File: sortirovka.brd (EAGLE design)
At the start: 160 x 100 mm, 19 parts, among them U1 MAX3485CSA, X1 PI3-CON, X2 MKDSN1,5/2-5,08, X3 MKDSN1,5/4-5,08, X4 MKDSN1,5/2-5,08

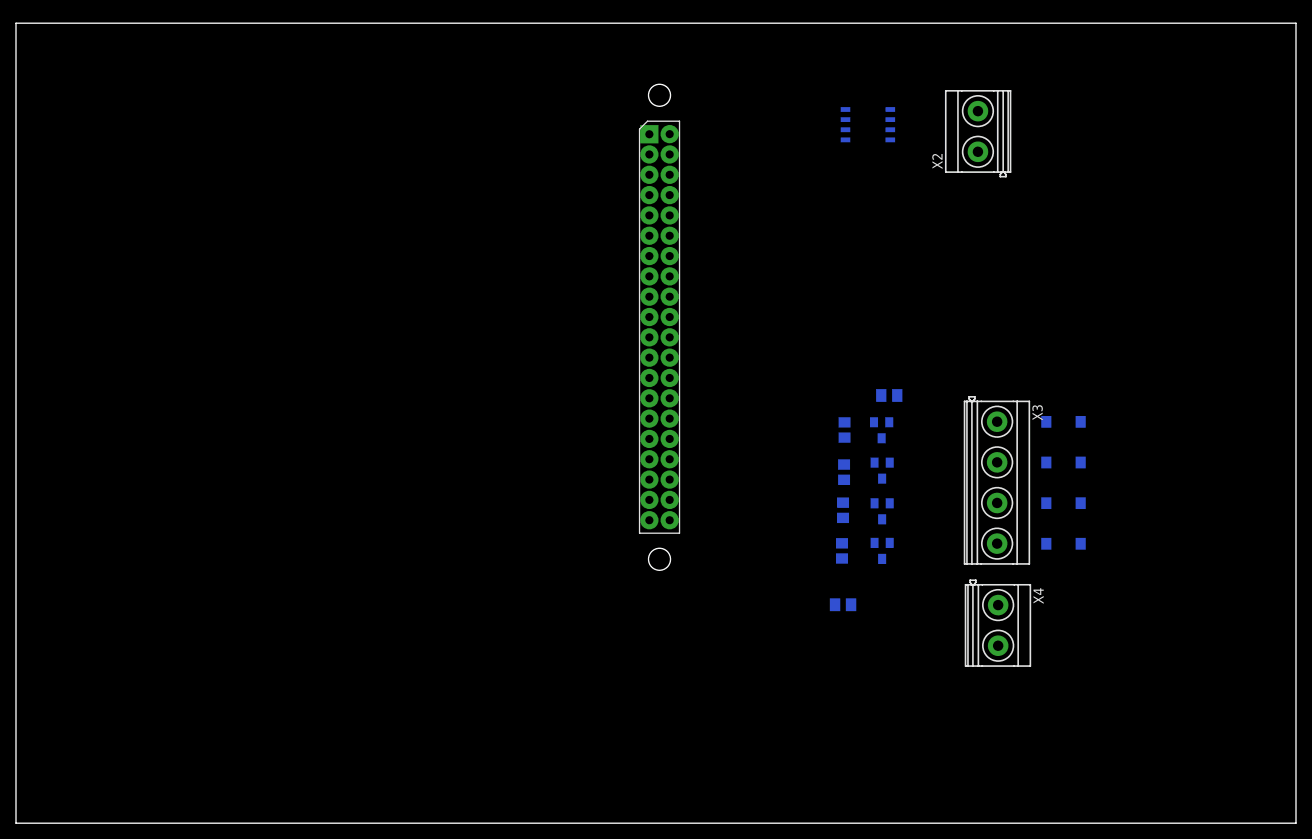
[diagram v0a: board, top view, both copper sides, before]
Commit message: rev1
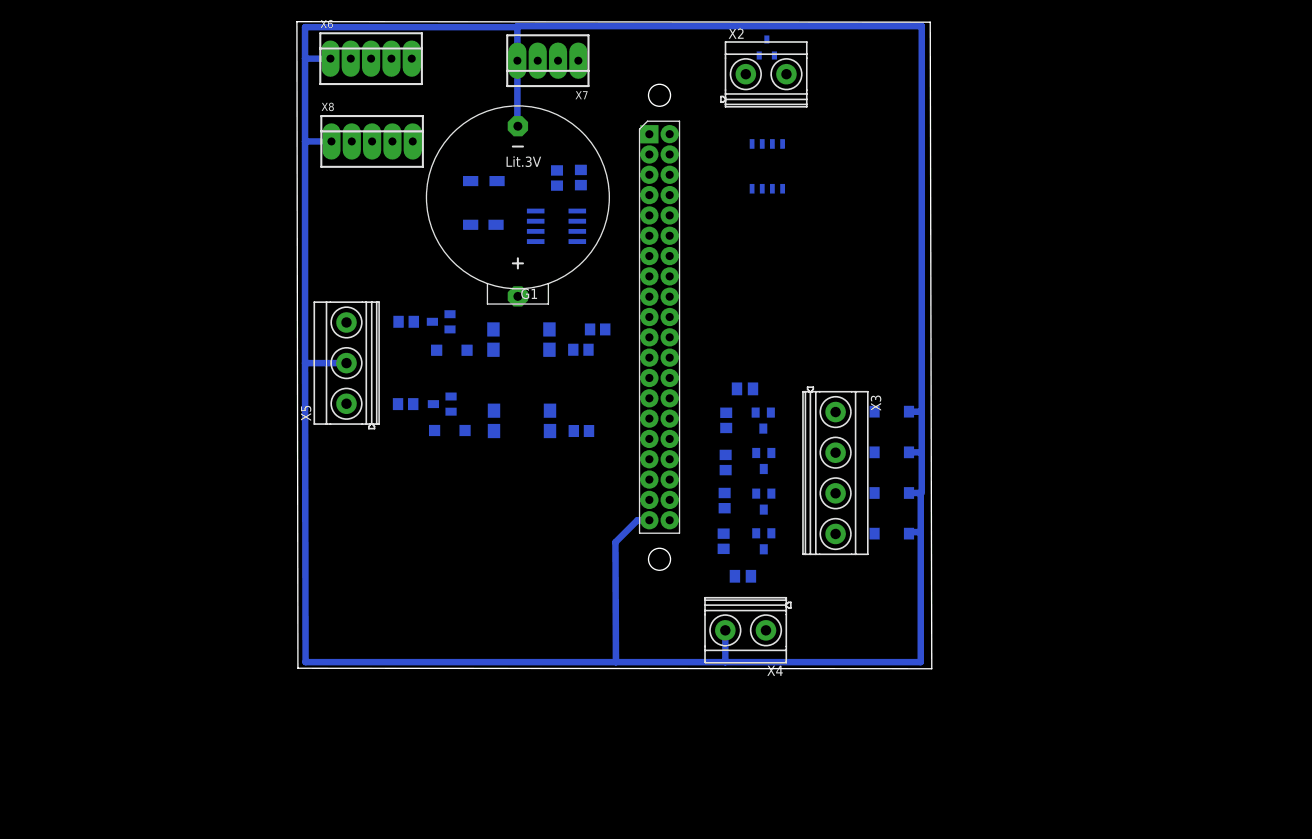
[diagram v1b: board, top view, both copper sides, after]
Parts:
- added D5, D6: BAV199, diode:SOT23
- added G1: CR2032H, MyLib:CR2032H
- added IC1: DS1307Z, MyLib:SOIC8
- added OC1, OC2: (no value), MyLib:SMD4
- added Q5: (no value), MyLib:MA306
- added R10, R11: 3k3, rcl:R0805
- added R5, R6: 10k, rcl:R0805
- added R7: 0, rcl:R0805
- added R8, R9: 100, rcl:R0805
- added U$1, U$2: NSI45020AT1GSOD-123, MyLib:SOD123
- added U$3: NUP2105LSOT23-R, MyLib:SOT23-R
- added X5: MKDSN1,5/3-5,08, con-phoenix-508:MKDSN1,5/3-5,08
- added X6, X8: 22-23-2051, con-molex:22-23-2051
- added X7: 22-23-2041, con-molex:22-23-2041
- R1, R2, R3, R4: value (none) -> 10k
- moved X4 31.6 mm to (91.2, 24.1), turned to 180 degrees
- moved X2 27.4 mm to (93.8, 93.6), turned to 0 degrees
- moved D1 21.5 mm to (109.5, 36.2)
- moved D2 21.5 mm to (109.5, 41.3)
- moved D3 21.5 mm to (109.5, 46.4)
- moved D4 21.5 mm to (109.5, 51.4)
- moved X3 20.2 mm to (102.4, 43.8)
- moved C2 18.1 mm to (91.1, 54.3), turned to 0 degrees
- moved Q1 14.8 mm to (93.5, 35.2)
- moved Q2 14.8 mm to (93.5, 40.2)
- moved Q3 14.8 mm to (93.5, 45.3)
- moved R1 14.8 mm to (88.5, 35.2)
- moved R2 14.8 mm to (88.6, 40.3)
- moved R4 14.8 mm to (88.8, 50.4)
- moved Q4 14.8 mm to (93.4, 50.3)
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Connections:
- new net +5V: IC1.8
- new net MISO: X1.P$21, X6.4, X8.4
- new net MOSI: X1.P$19, X6.5, X8.5
- new net N$14: R7.1, X1.P$1, X1.P$17
- new net N$15: OC2.4, R6.2, X1.P$31
- new net N$16: OC1.1, U$1.C
- new net N$17: OC2.1, U$2.C
- new net N$18: OC1.4, R5.2, X1.P$29
- new net N$19: D5.3, R8.1, U$1.A
- new net N$20: G1.+, IC1.3
- new net N$21: R8.2, X5.3
- new net N$22: R9.2, X5.1
- new net N$23: IC1.1, Q5.1
- new net N$24: D6.3, R9.1, U$2.A
- new net N$25: IC1.2, Q5.4
- new net N$26: IC1.6, R10.1, X1.P$5, X7.2
- new net N$27: IC1.5, R11.1, X1.P$3, X7.1
- new net SPI0: X1.P$24, X6.2
- new net SPI1: X1.P$26, X8.2
- new net SPI_CLK: X1.P$23, X6.3, X8.3
- net +24V: now also D5.2, D6.2
- net +3V3: now also OC1.3, OC2.3, R10.2, R11.2, R7.2, X7.3; no longer X1.P$1, X1.P$17
- net GND: now also D5.1, D6.1, G1.-, IC1.4, OC1.2, OC2.2, R5.1, R6.1, U$3.3, X1.P$14, X1.P$25, X5.2, X6.1, X7.4, X8.1
- net N$4: now also U$3.2, U1.6; no longer U1.7
- net N$5: now also U$3.1, U1.7; no longer U1.6
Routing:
- net GND: track 0.00 -> 367.8 mm
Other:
- board size 160 x 100 mm -> 79.4 x 80.9 mm
